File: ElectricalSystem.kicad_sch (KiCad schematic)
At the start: 15 parts, among them K1 HV+ Contactor, K2 HV- Contactor, K3 Array Main Contactor, K4 Array Precharge Contactor, K5 Motor Precharge Contactor, K6 Motor Contactor, M1 Mitsuba M2096-III Motor, SW3 Supp_Enable

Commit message: done except telemetry
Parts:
- added F2: 3A?, symbol Device:Fuse
- added R3: ???, symbol Device:R
- K6: value Motor Contactor -> Motor Main Contactor
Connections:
- net ARR_HV+: now also K3.L1
- net ArrayPreRes-: now also K5.L2, F2.2, R3.2
- net HV-: now also K2.L1
- net MTR_HV+: now also K6.L1
- net MotorPreRes+: now reaches K5.L1
- net MotorPreRes+: now also K6.L2, R3.1
- new net DC-DC-Converter/HV+: F2.1
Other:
- sheet VehicleControlUnit ports: added MotorPreReady, MotorPreSPI; removed none
- note added: "add dynamics + linpot (4x), environment (6x??), TPMS transceiver (4x), broker?"
- note added: "add e-stops"
- note removed: "add bus bar connections, e-stops"
- note removed: "add fuse - bus bar?"
- note removed: "add leader (+ wireless stuff), dynamics + linpot (4x), environment (6x??), TPMS transceiver (4x), broker?"
- note removed: "bus bar?"
- note removed: "change to separate precharge boards for BPS/VCU"
- moved on the sheet: F1, R1, R2

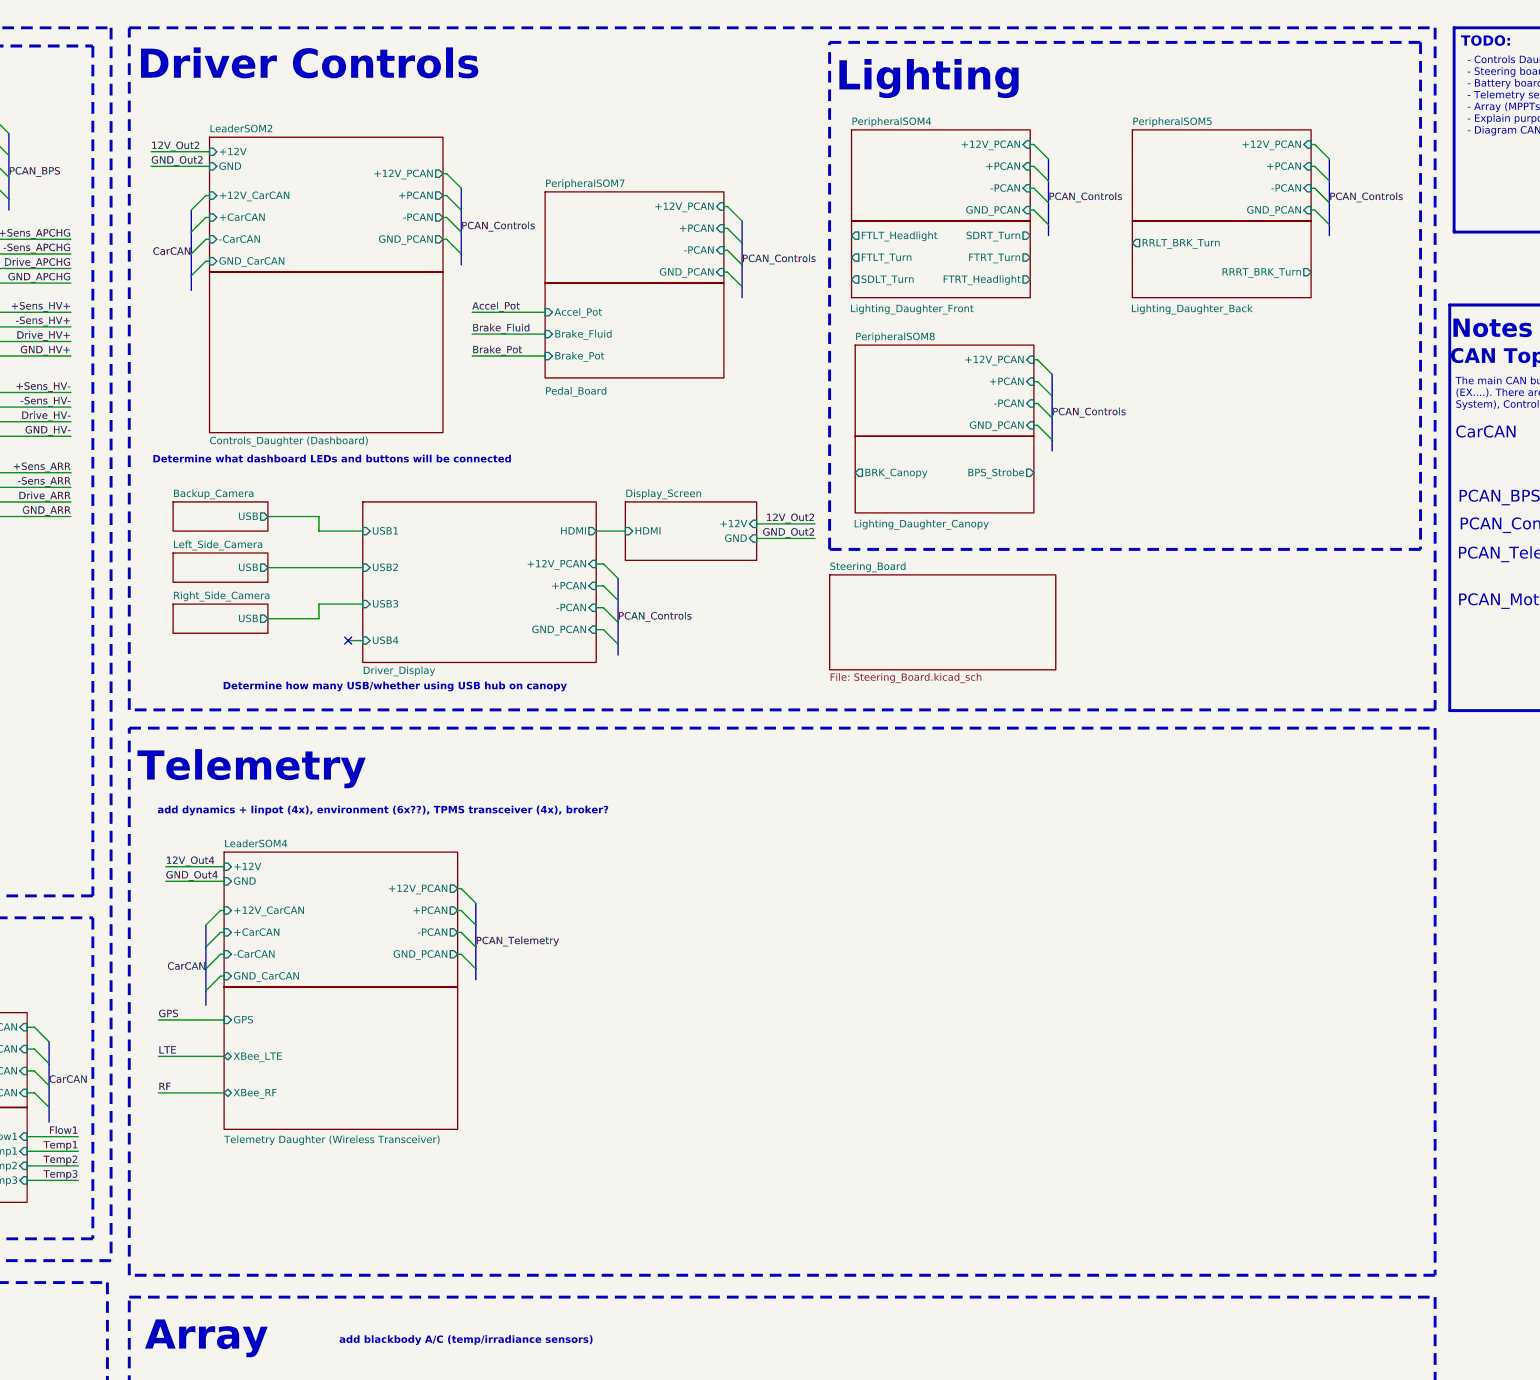
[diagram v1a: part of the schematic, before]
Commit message: steering
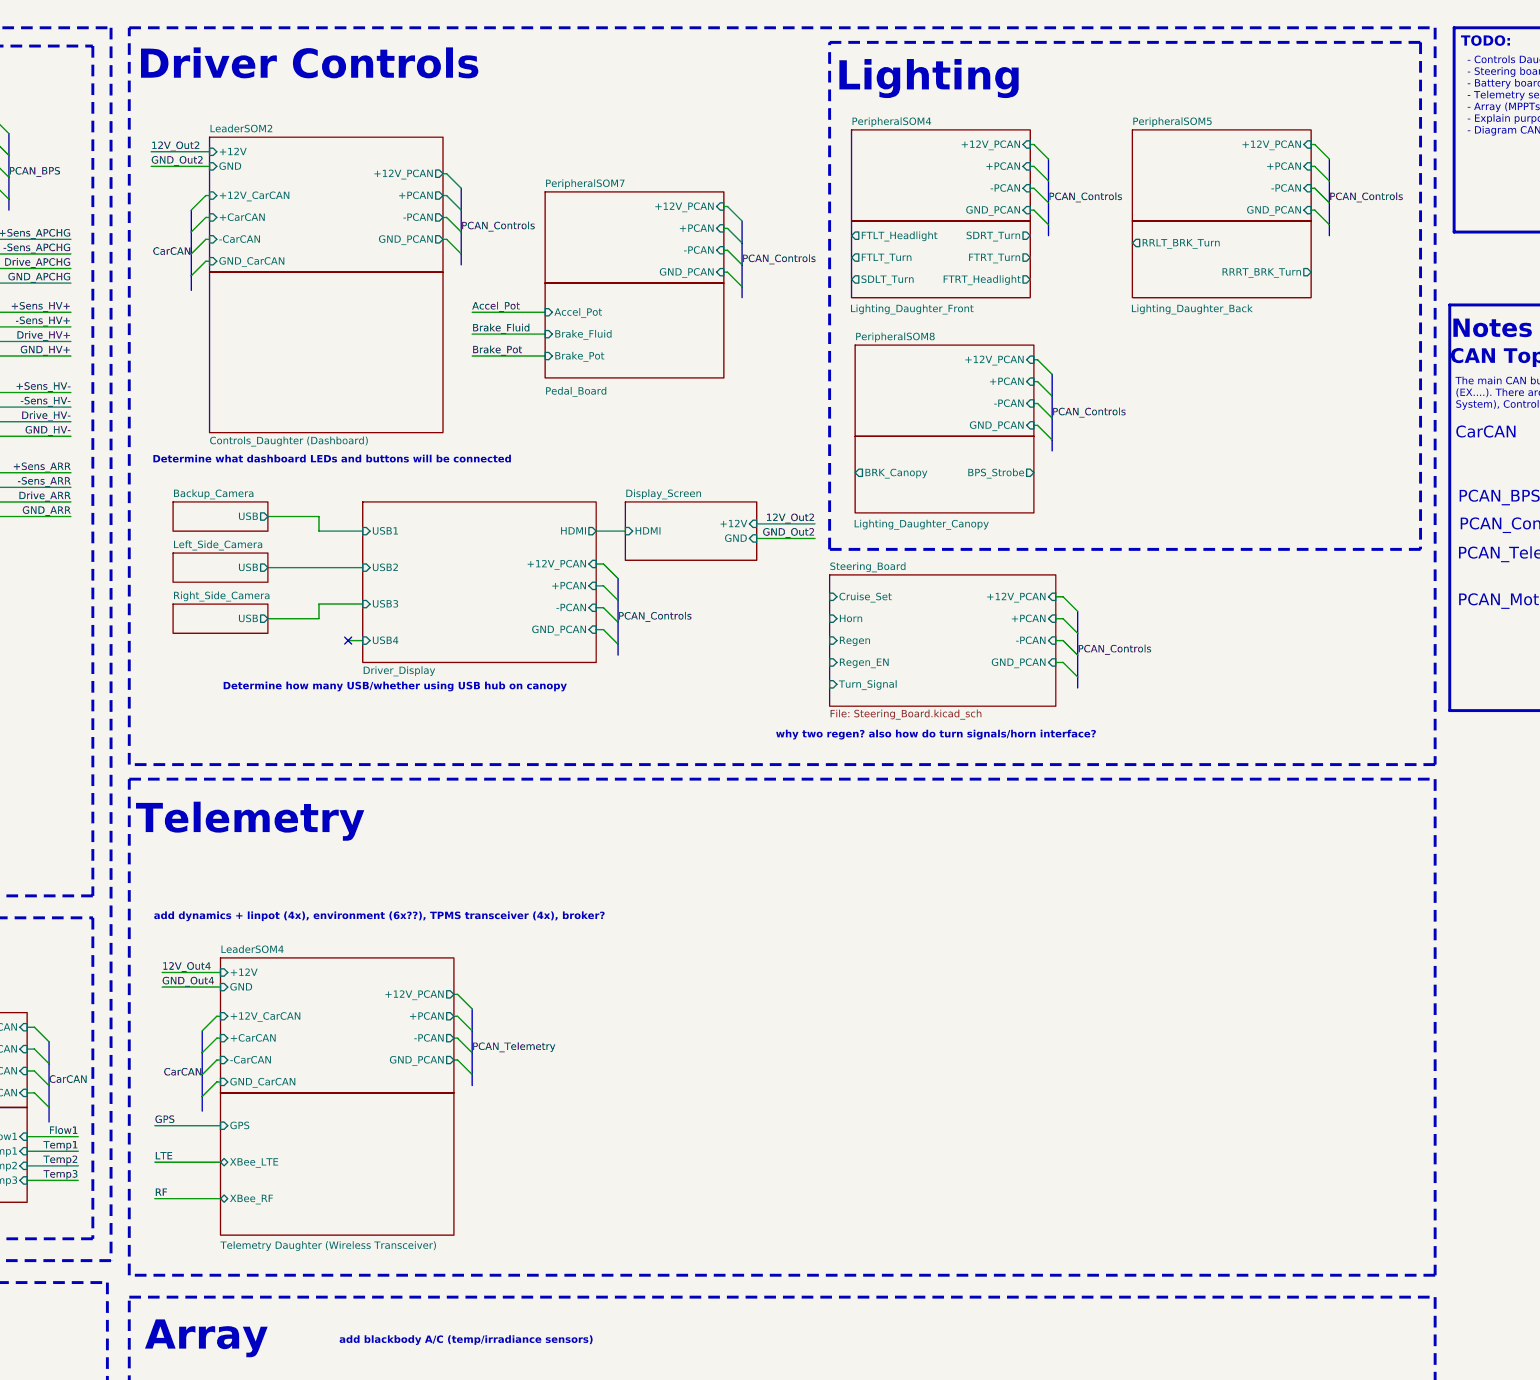
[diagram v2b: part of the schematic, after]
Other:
- sheet Steering_Board ports: added +12V_PCAN, +PCAN, -PCAN, Cruise_Set, GND_PCAN, Horn, Regen, Regen_EN, Turn_Signal; removed none
- note added: "why two regen? also how do turn signals/horn interface?"
